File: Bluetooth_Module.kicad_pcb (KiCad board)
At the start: 2 copper layers, 96.8 x 104.7 mm, 31 parts, among them J1 Conn_01x04_Pin, Q1 STN3NF06, Q2 BC817, Q3 BC817, Q4 STN3NF06, Q5 BC817, Q6 STN3NF06, U1 ESP32-C3-DevKitM-1

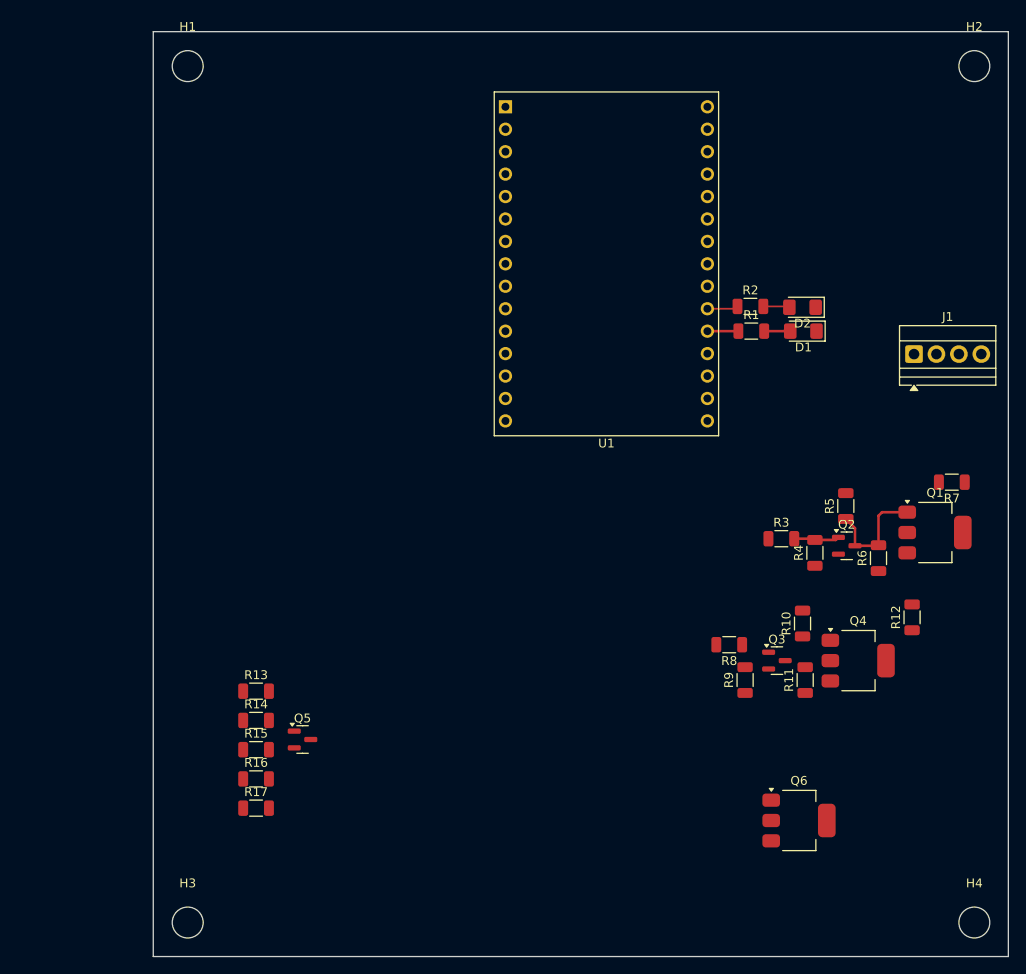
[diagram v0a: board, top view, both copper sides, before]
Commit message: Lesson 4 - Power Supply
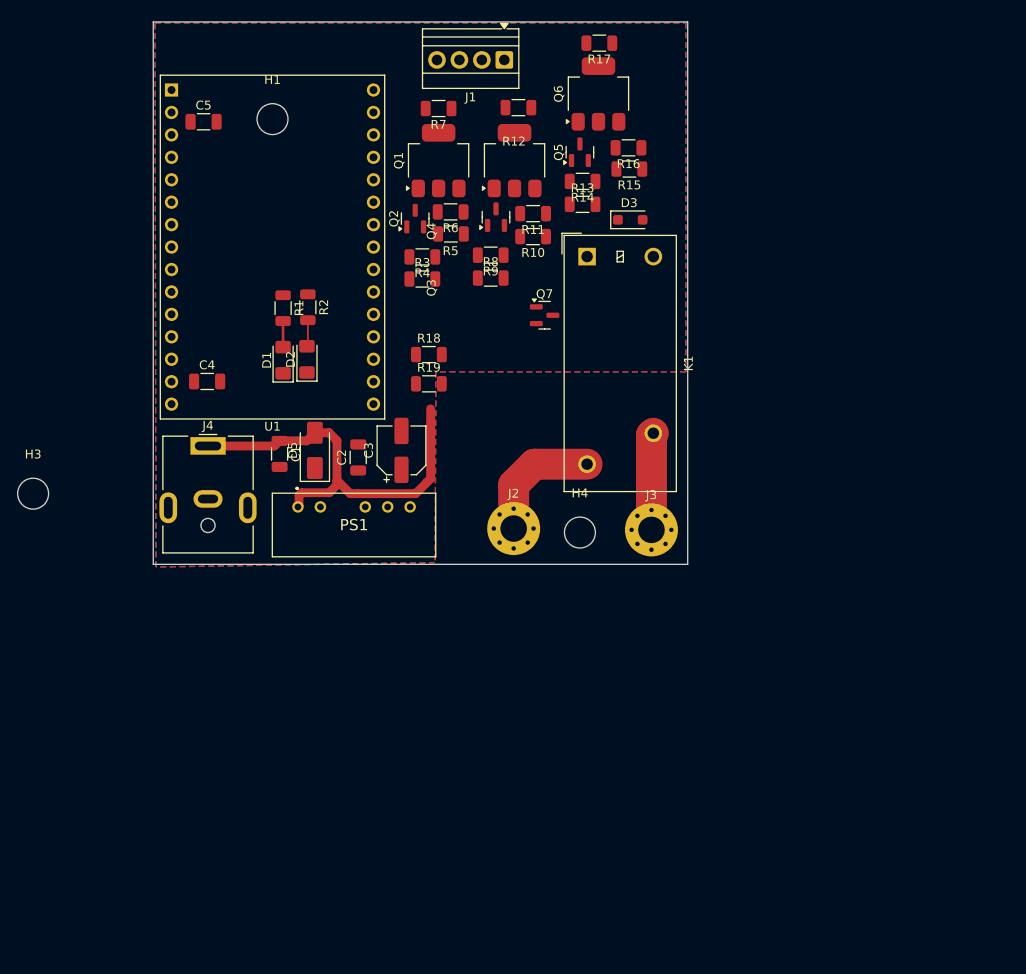
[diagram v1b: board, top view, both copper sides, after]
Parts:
- removed H2: MountingHole, MountingHole:MountingHole_3.5mm
- added C1: 100n/25V, Capacitor_SMD:C_1206_3216Metric, F.Cu at (103.4, 100.9)
- added C2: 100n/25V, Capacitor_SMD:C_1206_3216Metric, F.Cu at (112.3, 101.3)
- added C3: 22uF/35V, Capacitor_SMD:CP_Elec_5x5.8, F.Cu at (117.2, 100.5)
- added C4: 100n/25V, Capacitor_SMD:C_1206_3216Metric, F.Cu at (95.2, 92.7)
- added C5: 100n/25V, Capacitor_SMD:C_1206_3216Metric, F.Cu at (94.8, 63.3)
- added D3: D, Diode_SMD:D_SOD-123F, F.Cu at (143.1, 74.4)
- added D5: D_TVS_12V, Diode_SMD:D_SMA, F.Cu at (107.4, 100.5)
- added J2: Conn_01x01_Socket, MountingHole:MountingHole_3mm_Pad_Via, F.Cu at (129.9, 109.3)
- added J3: Conn_01x01_Socket, MountingHole:MountingHole_3mm_Pad_Via, F.Cu at (145.5, 109.5)
- added J4: Jack-DC, Connector_BarrelJack:BarrelJack_CUI_PJ-063AH_Horizontal, F.Cu at (95.3, 100.0)
- added K1: G2RL-1A-H, Relay_THT:Relay_SPST_Omron_G2RL-1A, F.Cu at (138.2, 78.6)
- added PS1: DPU01N-15, SPU01M:DPU01N15, F.Cu at (105.5, 106.9)
- added Q7: BC817, Package_TO_SOT_SMD:SOT-23, F.Cu at (133.4, 85.2)
- added R18: 1k, Resistor_SMD:R_1206_3216Metric, F.Cu at (120.3, 89.7)
- added R19: 10k, Resistor_SMD:R_1206_3216Metric, F.Cu at (120.3, 93.0)
- moved R17 94.9 mm to (139.6, 54.4), turned to 180 degrees
- moved Q6 85.3 mm to (139.5, 60.1), turned to 90 degrees
- moved R16 83.0 mm to (142.9, 66.2), turned to 180 degrees
- moved R15 78.1 mm to (143.0, 68.7), turned to 180 degrees
- moved Q5 73.5 mm to (137.4, 66.8), turned to 90 degrees
- moved R12 72.9 mm to (130.4, 61.7), turned to 180 degrees
- moved R7 71.9 mm to (121.4, 61.8)
- moved R14 71.3 mm to (137.7, 70.0), turned to 180 degrees
- moved Q1 70.2 mm to (121.4, 67.7), turned to 90 degrees
- moved Q4 68.7 mm to (130.0, 67.7), turned to 90 degrees
- moved R13 66.4 mm to (137.7, 72.7)
- moved H4 62.8 mm to (137.4, 109.8)
- moved R6 62.3 mm to (122.8, 73.5), turned to 180 degrees
- moved Q2 61.3 mm to (118.8, 74.3), turned to 90 degrees
- moved R11 61.1 mm to (132.1, 73.7), turned to 180 degrees
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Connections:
- net Net-(U1-5V-Pad13) renamed +5V
- R2 pad 1: Net-(U1-IO5) -> unconnected-(R2-Pad1)
- U1 pad 1: Net-(U1-GND-Pad1) -> GND
- U1 pad 12: Net-(U1-GND-Pad1) -> GND
- U1 pad 15: Net-(U1-GND-Pad1) -> GND
- U1 pad 16: Net-(U1-GND-Pad1) -> GND
- U1 pad 19: Net-(U1-GND-Pad1) -> GND
- U1 pad 2: Net-(U1-3V3-Pad2) -> +3V3
- U1 pad 21: Net-(U1-IO5) -> LED_R
- U1 pad 22: LED_R -> LED_G
- U1 pad 23: LED_G -> LED_B
- U1 pad 24: Net-(U1-GND-Pad1) -> GND
- U1 pad 25: LED_B -> unconnected-(U1-IO8-Pad25)
- U1 pad 27: Net-(U1-GND-Pad1) -> GND
- U1 pad 3: Net-(U1-3V3-Pad2) -> +3V3
- U1 pad 30: Net-(U1-GND-Pad1) -> GND
- U1 pad 6: Net-(U1-GND-Pad1) -> GND
- U1 pad 8: Net-(U1-GND-Pad1) -> GND
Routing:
- net +12V: track 0.00 -> 46.6 mm
- net Net-(J2-Pin_1): track 0.00 -> 14.2 mm
- net Net-(Q1-G): track 12.9 -> 0.00 mm
- net Net-(J3-Pin_1): track 0.00 -> 11.0 mm
- net Net-(Q2-B): track 5.18 -> 0.00 mm
- net Net-(U1-IO5): track 3.52 -> 0.00 mm
- net Net-(U1-IO4): track 3.51 -> 0.00 mm
- added copper zone on B.Cu, net GND
- added copper zone on F.Cu, net GND
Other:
- board size 96.8 x 104.7 mm -> 60.5 x 61.4 mm
- board text added: "For 230 VAC appliances (IEC 60335-1 typical case): Working voltage ≈ 250 V CTI ≥ 400 (FR-4 often MG II) Pollution Degree 2 Required reinforced creepage = 5.0 mm"
- board text added: "Obudowa Z54 KRADEX"
- board text removed: "Obudowa Z59J PSKRADEX"
